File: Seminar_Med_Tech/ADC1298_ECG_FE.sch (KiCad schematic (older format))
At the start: 54 parts, among them J6 DB15_F-RA

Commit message: Update
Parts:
- D1, D10, D2, D3, D4, D5, D6, D7, D8, D9: footprint Diodes_SMD:D_SC-80_HandSoldering -> Diodes_SMD:D_SOD-123
- PSK4: footprint Pin_Headers:Pin_Header_Straight_1x03_Pitch2.54mm -> Pin_Headers:Pin_Header_Straight_1x02_Pitch2.54mm
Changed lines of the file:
@@
 F 0 "D1" H 3400 1075 50  0000 C CNN
 F 1 "D" H 3400 875 50  0000 C CNN
-F 2 "Diodes_SMD:D_SC-80_HandSoldering" H 3400 975 50  0001 C CNN
+F 2 "Diodes_SMD:D_SOD-123" H 3400 975 50  0001 C CNN
 F 3 "" H 3400 975 50  0001 C CNN
 	1    3400 975
@@
 F 0 "D5" H 6175 1100 50  0000 C CNN
 F 1 "D" H 6175 900 50  0000 C CNN
-F 2 "Diodes_SMD:D_SC-80_HandSoldering" H 6175 1000 50  0001 C CNN
+F 2 "Diodes_SMD:D_SOD-123" H 6175 1000 50  0001 C CNN
 F 3 "" H 6175 1000 50  0001 C CNN
 	1    6175 1000
@@
 F 0 "D10" H 9175 1050 50  0000 C CNN
 F 1 "D" H 9175 850 50  0000 C CNN
-F 2 "Diodes_SMD:D_SC-80_HandSoldering" H 9175 950 50  0001 C CNN
+F 2 "Diodes_SMD:D_SOD-123" H 9175 950 50  0001 C CNN
 F 3 "" H 9175 950 50  0001 C CNN
 	1    9175 950
@@
 F 0 "D2" H 3625 2500 50  0000 C CNN
 F 1 "D" H 3625 2300 50  0000 C CNN
-F 2 "Diodes_SMD:D_SC-80_HandSoldering" H 3625 2400 50  0001 C CNN
+F 2 "Diodes_SMD:D_SOD-123" H 3625 2400 50  0001 C CNN
 F 3 "" H 3625 2400 50  0001 C CNN
 	1    3625 2400
@@
 F 0 "D6" H 6200 2525 50  0000 C CNN
 F 1 "D" H 6200 2325 50  0000 C CNN
-F 2 "Diodes_SMD:D_SC-80_HandSoldering" H 6200 2425 50  0001 C CNN
+F 2 "Diodes_SMD:D_SOD-123" H 6200 2425 50  0001 C CNN
 F 3 "" H 6200 2425 50  0001 C CNN
 	1    6200 2425
@@
 F 0 "D9" H 9025 2500 50  0000 C CNN
 F 1 "D" H 9025 2300 50  0000 C CNN
-F 2 "Diodes_SMD:D_SC-80_HandSoldering" H 9025 2400 50  0001 C CNN
+F 2 "Diodes_SMD:D_SOD-123" H 9025 2400 50  0001 C CNN
 F 3 "" H 9025 2400 50  0001 C CNN
 	1    9025 2400
@@
 F 0 "D7" H 8325 4175 50  0000 C CNN
 F 1 "D" H 8325 3975 50  0000 C CNN
-F 2 "Diodes_SMD:D_SC-80_HandSoldering" H 8325 4075 50  0001 C CNN
+F 2 "Diodes_SMD:D_SOD-123" H 8325 4075 50  0001 C CNN
 F 3 "" H 8325 4075 50  0001 C CNN
 	1    8325 4075
@@
 F 0 "D8" H 9000 5225 50  0000 C CNN
 F 1 "D" H 9000 5025 50  0000 C CNN
-F 2 "Diodes_SMD:D_SC-80_HandSoldering" H 9000 5125 50  0001 C CNN
+F 2 "Diodes_SMD:D_SOD-123" H 9000 5125 50  0001 C CNN
 F 3 "" H 9000 5125 50  0001 C CNN
 	1    9000 5125
@@
 F 0 "D3" H 5125 5050 50  0000 C CNN
 F 1 "D" H 5125 4850 50  0000 C CNN
-F 2 "Diodes_SMD:D_SC-80_HandSoldering" H 5125 4950 50  0001 C CNN
+F 2 "Diodes_SMD:D_SOD-123" H 5125 4950 50  0001 C CNN
 F 3 "" H 5125 4950 50  0001 C CNN
 	1    5125 4950
@@
 F 0 "D4" H 5400 6075 50  0000 C CNN
 F 1 "D" H 5400 5875 50  0000 C CNN
-F 2 "Diodes_SMD:D_SC-80_HandSoldering" H 5400 5975 50  0001 C CNN
+F 2 "Diodes_SMD:D_SOD-123" H 5400 5975 50  0001 C CNN
 F 3 "" H 5400 5975 50  0001 C CNN
 	1    5400 5975
@@
 F 0 "PSK4" H 675 5225 50  0000 C CNN
 F 1 "CONN_01X02" V 800 5050 50  0000 C CNN
-F 2 "Pin_Headers:Pin_Header_Straight_1x03_Pitch2.54mm" H 700 5050 50  0001 C CNN
+F 2 "Pin_Headers:Pin_Header_Straight_1x02_Pitch2.54mm" H 700 5050 50  0001 C CNN
 F 3 "" H 700 5050 50  0001 C CNN
 	1    700  5050

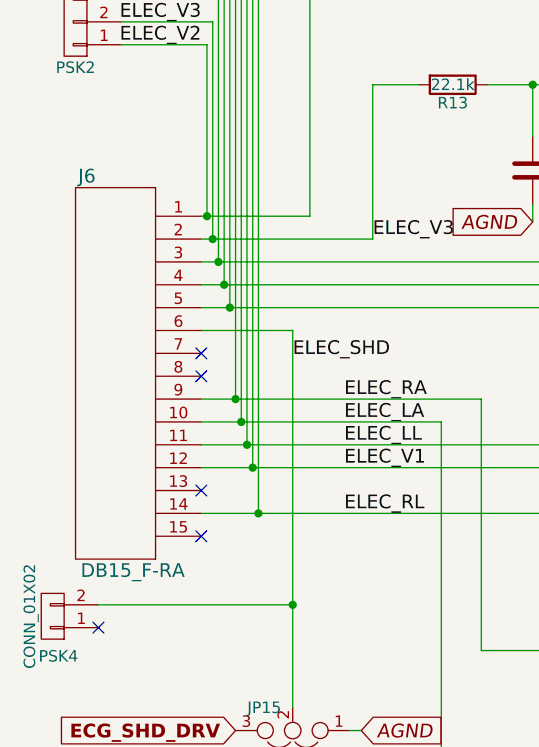
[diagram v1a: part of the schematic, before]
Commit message: Update from develop
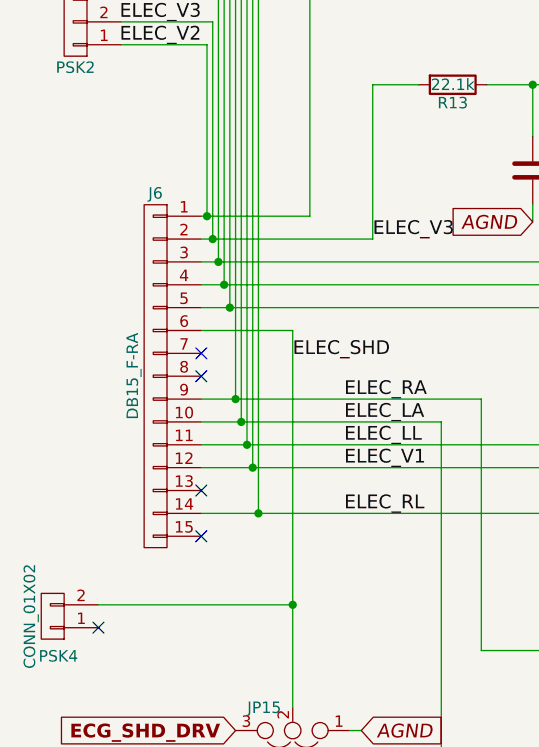
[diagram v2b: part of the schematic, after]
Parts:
- removed J6: DB15_F-RA, Connectors:DB15FC, symbol DB15_F-RA
- added J6: DB15_F-RA, symbol CONN_01X15
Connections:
- net ELEC_LA: now also J6.10 (P10)
- net ELEC_LL: now also J6.11 (P11)
- net ELEC_RA: now also J6.9 (P9)
- net ELEC_RL: now also J6.14 (P14)
- net ELEC_SHD: now also J6.6 (P6)
- net ELEC_V1: now also J6.12 (P12)
- net ELEC_V2: now also J6.1 (P1)
- net ELEC_V3: now also J6.2 (P2)
- net ELEC_V4: now also J6.3 (P3)
- net ELEC_V5: now also J6.4 (P4)
- net ELEC_V6: now also J6.5 (P5)
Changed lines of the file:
@@
 $EndDescr
-$Comp
-L DB15_F-RA J6
-U 1 1 59454B8D
-P 450 4975
-F 0 "J6" H 850 6825 60  0000 C CNN
-F 1 "DB15_F-RA" H 1050 5100 60  0000 C CNN
-F 2 "Connectors:DB15FC" H 450 4975 60  0001 C CNN
-F 3 "" H 450 4975 60  0001 C CNN
-	1    450  4975
-	1    0    0    -1
-$EndComp
 $Comp
 L R R9
@@
 Text Label 1350 1950 2    60   ~ 0
 ELEC_LA
+$Comp
+L CONN_01X15 J6
+U 1 1 594BFFB9
+P 1150 4000
+F 0 "J6" H 1150 4800 50  0000 C CNN
+F 1 "DB15_F-RA" V 1250 4000 50  0000 C CNN
+F 2 "" H 1150 4000 50  0001 C CNN
+F 3 "" H 1150 4000 50  0001 C CNN
+	1    1150 4000
+	-1   0    0    -1
+$EndComp
 $EndSCHEMATC

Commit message: Update
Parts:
- J6: footprint (none) -> Connectors:DB15FC
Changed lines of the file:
@@
 F 0 "J6" H 1150 4800 50  0000 C CNN
 F 1 "DB15_F-RA" V 1250 4000 50  0000 C CNN
-F 2 "" H 1150 4000 50  0001 C CNN
+F 2 "Connectors:DB15FC" H 1150 4000 50  0001 C CNN
 F 3 "" H 1150 4000 50  0001 C CNN
 	1    1150 4000
